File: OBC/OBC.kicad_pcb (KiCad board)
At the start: 2 copper layers, 93 x 93 mm, 23 parts, among them J101 Modos de operación, J102 PMS-Raspi, J103 Conector UART, J104 Raspi-TRU, U101 RASPBERRY_PI_ZERO_2_W, U102 BMP280, U201 ADS1115IDGS

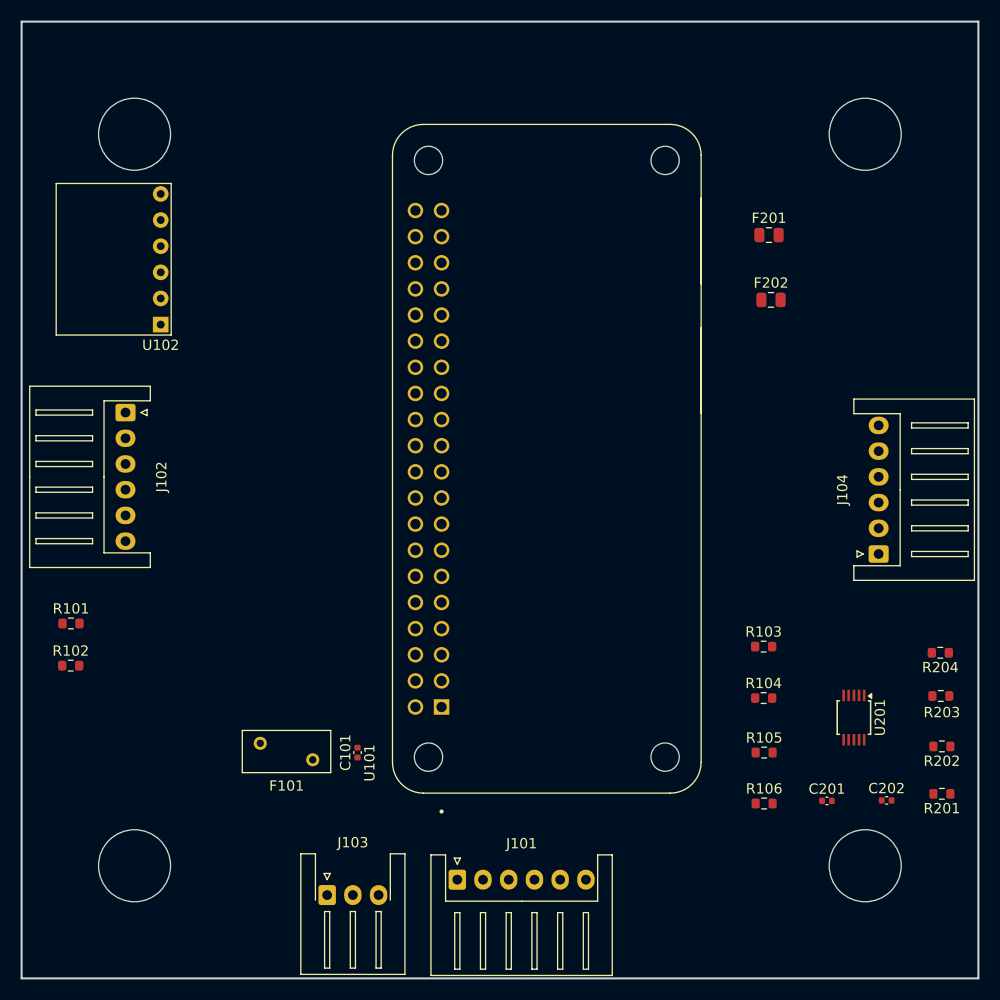
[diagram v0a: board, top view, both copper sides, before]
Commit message: Propone disposicion pcb
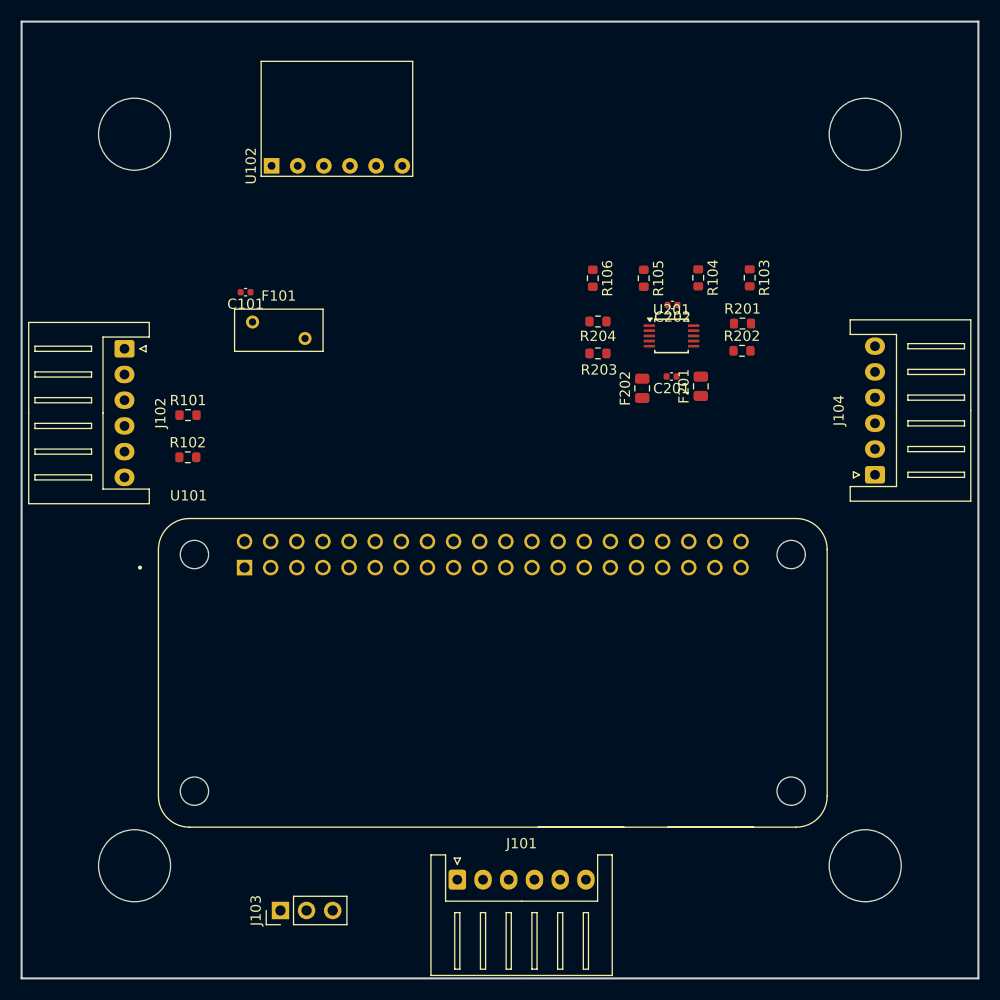
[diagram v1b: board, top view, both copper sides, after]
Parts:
- J103: footprint Connector_JST:JST_XH_S3B-XH-A-1_1x03_P2.50mm_Horizontal -> Connector_PinHeader_2.54mm:PinHeader_1x03_P2.54mm_Vertical
- moved R106 53.7 mm to (167.0, 57.5), turned to -90 degrees
- moved C202 52.5 mm to (174.8, 60.0), turned to 180 degrees
- moved R201 49.6 mm to (181.6, 61.9), turned to 0 degrees
- moved R105 47.6 mm to (172.0, 57.5), turned to -90 degrees
- moved R203 47.1 mm to (167.5, 64.8)
- moved R204 46.3 mm to (167.5, 61.6)
- moved C101 46.1 mm to (133.3, 58.8), turned to 180 degrees
- moved C201 43.9 mm to (174.7, 67.0), turned to 180 degrees
- moved R202 43.1 mm to (181.5, 64.5), turned to 0 degrees
- moved F101 43.0 mm to (133.9, 61.7), turned to 0 degrees
- moved R104 41.3 mm to (177.3, 57.4), turned to -90 degrees
- moved U201 41.1 mm to (174.7, 63.0), turned to 0 degrees
- moved R103 35.9 mm to (182.3, 57.4), turned to -90 degrees
- moved R101 23.2 mm to (127.7, 70.8)
- moved R102 23.2 mm to (127.7, 74.8)
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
